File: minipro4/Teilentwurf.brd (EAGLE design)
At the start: 105.1 x 94.6 mm, 91 parts, among them IC1 MEGA8-P, IC2 FT232RL_ADAPTER, IC3 78L08Z, IC4 4051N, IC5 TL082P, IC6 4051N, IC7 TL082P, J1 HOHLSTECKER, Q2 BS170, Q3 BS170, Q4 BS170, Q6 IRF4905, X1 , X2 CON_COAX

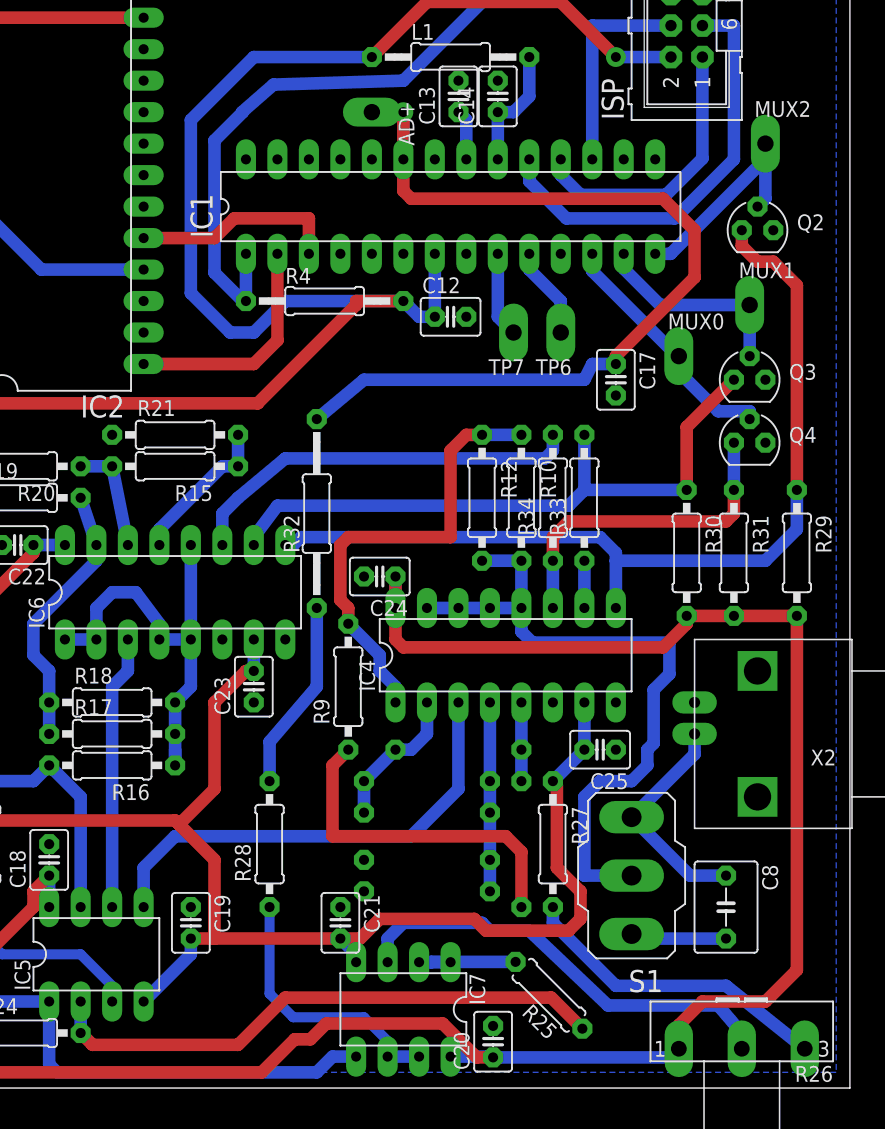
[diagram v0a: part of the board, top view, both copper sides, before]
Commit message: Winkel überarbeitet
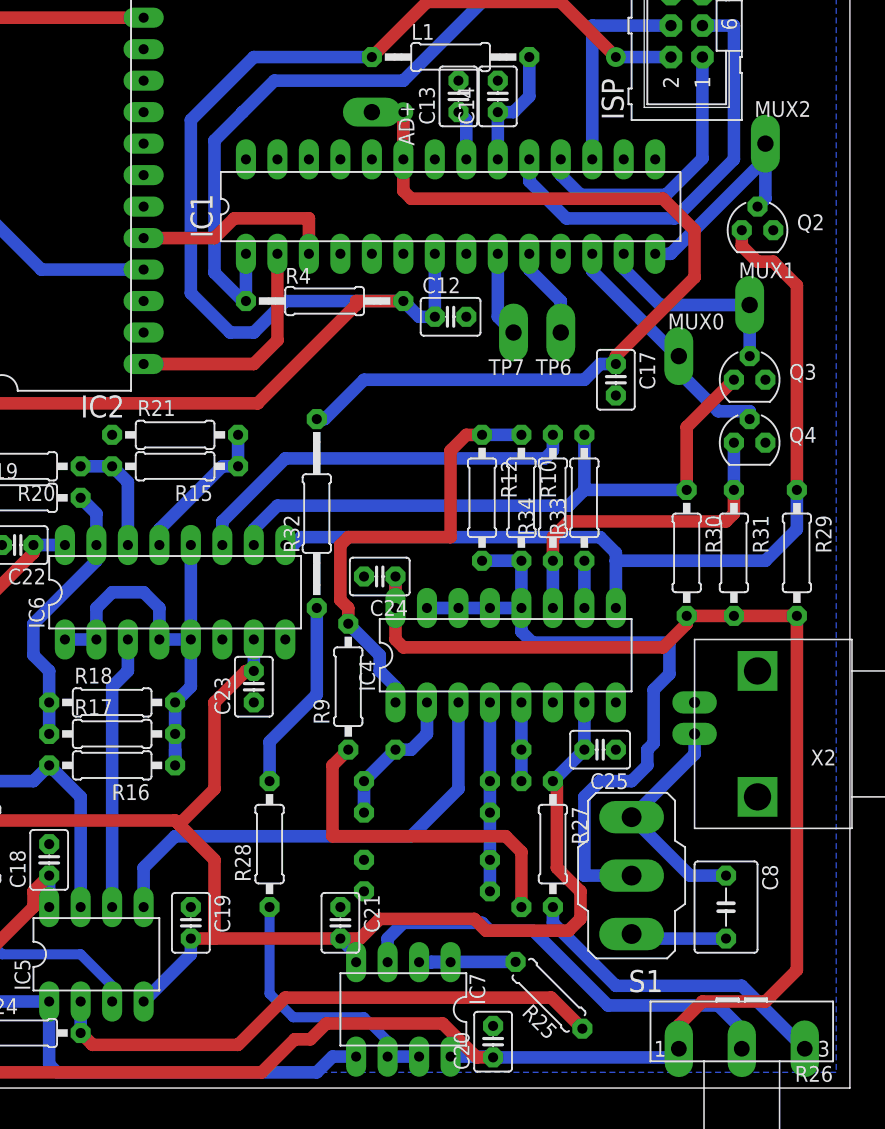
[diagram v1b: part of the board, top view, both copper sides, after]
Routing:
- net N$23: track 35.3 -> 35.9 mm
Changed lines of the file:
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@@
 </class>
 </classes>
-<designrules name="DesignRules_Grounplane">
+<designrules name="DesignRules_Grounplane *">
 <description language="de">&lt;b&gt;EAGLE Design Rules&lt;/b&gt;
 &lt;p&gt;
@@
 <param name="dpGapFactor" value="2.5"/>
 <param name="checkGrid" value="0"/>
-<param name="checkAngle" value="0"/>
+<param name="checkAngle" value="1"/>
 <param name="checkFont" value="1"/>
 <param name="checkRestrict" value="1"/>
@@
 <contactref element="C17" pad="1"/>
 <wire x1="92.71" y1="67.31" x2="92.71" y2="63.5" width="1.016" layer="1"/>
-<wire x1="62.23" y1="52.07" x2="66.04" y2="55.245" width="1.016" layer="16"/>
 <wire x1="66.04" y1="55.245" x2="83.82" y2="55.245" width="1.016" layer="16"/>
-<wire x1="83.82" y1="55.245" x2="84.455" y2="56.515" width="1.016" layer="16"/>
-<wire x1="84.455" y1="56.515" x2="86.36" y2="56.515" width="1.016" layer="16"/>
 <wire x1="86.36" y1="56.515" x2="86.36" y2="57.15" width="1.016" layer="1"/>
 <wire x1="86.36" y1="57.15" x2="92.71" y2="63.5" width="1.016" layer="1"/>
@@
 <wire x1="69.215" y1="73.025" x2="69.215" y2="76.835" width="1.016" layer="1"/>
 <via x="69.215" y="76.835" extent="1-16" drill="0.8" shape="square"/>
+<wire x1="66.04" y1="55.245" x2="62.865" y2="52.07" width="1.016" layer="16"/>
+<wire x1="62.865" y1="52.07" x2="62.23" y2="52.07" width="1.016" layer="16"/>
+<wire x1="86.36" y1="56.515" x2="85.09" y2="56.515" width="1.016" layer="16"/>
+<wire x1="85.09" y1="56.515" x2="83.82" y2="55.245" width="1.016" layer="16"/>
 </signal>
 <signal name="MUX0">
@@
 <wire x1="56.2645" y1="61.595" x2="53.975" y2="63.8845" width="1.016" layer="16"/>
 <wire x1="53.975" y1="63.8845" x2="53.975" y2="74.5455" width="1.016" layer="16"/>
-<wire x1="53.975" y1="74.5455" x2="56.2645" y2="76.835" width="1.016" layer="16"/>
 <wire x1="78.74" y1="88.9" x2="91.549" y2="88.9" width="1.016" layer="16"/>
 <wire x1="91.549" y1="88.9" x2="93.345" y2="87.104" width="1.016" layer="16"/>
 <wire x1="93.345" y1="87.104" x2="93.345" y2="86.36" width="1.016" layer="16"/>
 <wire x1="56.2645" y1="76.835" x2="56.1975" y2="76.835" width="1.016" layer="16"/>
-<wire x1="56.1975" y1="76.835" x2="58.7375" y2="79.0575" width="1.016" layer="16"/>
-<wire x1="58.7375" y1="79.0575" x2="69.215" y2="79.375" width="1.016" layer="16"/>
 <wire x1="69.215" y1="79.375" x2="78.74" y2="88.9" width="1.016" layer="16"/>
+<wire x1="69.215" y1="79.375" x2="58.8045" y2="79.375" width="1.016" layer="16"/>
+<wire x1="58.8045" y1="79.375" x2="53.975" y2="74.5455" width="1.016" layer="16"/>
+<wire x1="53.975" y1="74.5455" x2="56.1975" y2="76.835" width="0" layer="19" extent="16-16"/>
 </signal>
 <signal name="N$5">
@@
 <contactref element="IC6" pad="10"/>
 <contactref element="R33" pad="2"/>
-<wire x1="57.15" y1="41.91" x2="57.15" y2="42.545" width="1.016" layer="16"/>
-<wire x1="57.15" y1="42.545" x2="59.055" y2="45.085" width="1.016" layer="16"/>
 <wire x1="59.055" y1="45.085" x2="82.55" y2="45.085" width="1.016" layer="16"/>
 <wire x1="82.55" y1="45.085" x2="83.82" y2="46.355" width="1.016" layer="16"/>
 <wire x1="83.82" y1="46.355" x2="83.82" y2="50.8" width="1.016" layer="16"/>
 <wire x1="92.075" y1="46.355" x2="83.82" y2="46.355" width="1.016" layer="16"/>
+<wire x1="57.15" y1="41.91" x2="57.15" y2="43.18" width="1.016" layer="16"/>
+<wire x1="57.15" y1="43.18" x2="59.055" y2="45.085" width="1.016" layer="16"/>
 </signal>
 <signal name="MUX2*">
@@
 <contactref element="IC6" pad="14"/>
 <wire x1="43.18" y1="48.26" x2="45.72" y2="48.26" width="1.016" layer="16"/>
-<wire x1="45.72" y1="48.26" x2="46.99" y2="41.91" width="1.016" layer="16"/>
+<wire x1="46.99" y1="41.91" x2="46.99" y2="46.99" width="1.016" layer="16"/>
+<wire x1="46.99" y1="46.99" x2="45.72" y2="48.26" width="1.016" layer="16"/>
 </signal>
 <signal name="N$33">
@@
 <contactref element="R18" pad="1"/>
 <contactref element="IC6" pad="15"/>
-<wire x1="43.18" y1="45.72" x2="44.45" y2="41.91" width="1.016" layer="16"/>
 <wire x1="40.64" y1="29.21" x2="40.64" y2="26.67" width="1.016" layer="16"/>
 <wire x1="40.64" y1="29.21" x2="40.64" y2="31.75" width="1.016" layer="16"/>
@@
 <wire x1="39.37" y1="35.56" x2="44.45" y2="40.64" width="1.016" layer="16"/>
 <wire x1="44.45" y1="40.64" x2="44.45" y2="41.91" width="1.016" layer="16"/>
+<wire x1="44.45" y1="41.91" x2="44.45" y2="44.45" width="1.016" layer="16"/>
+<wire x1="44.45" y1="44.45" x2="43.18" y2="45.72" width="1.016" layer="16"/>
 </signal>
 <signal name="N$34">
@@
 <wire x1="81.28" y1="12.7" x2="81.28" y2="11.43" width="1.016" layer="16"/>
 <wire x1="81.28" y1="11.43" x2="86.36" y2="6.35" width="1.016" layer="16"/>
-<wire x1="95.25" y1="6.35" x2="101.6" y2="1.27" width="1.016" layer="16"/>
-<wire x1="86.36" y1="6.35" x2="95.25" y2="6.35" width="1.016" layer="16"/>
+<wire x1="86.36" y1="6.35" x2="96.52" y2="6.35" width="1.016" layer="16"/>
+<wire x1="96.52" y1="6.35" x2="101.6" y2="1.27" width="1.016" layer="16"/>
 </signal>
 <signal name="N$39">
@@
 <wire x1="67.945" y1="8.255" x2="67.945" y2="10.16" width="1.016" layer="16"/>
 <wire x1="67.945" y1="10.16" x2="69.215" y2="11.43" width="1.016" layer="16"/>
-<wire x1="96.52" y1="1.27" x2="96.52" y2="2.54" width="1.016" layer="16"/>
-<wire x1="96.52" y1="2.54" x2="94.615" y2="4.7625" width="1.016" layer="16"/>
+<wire x1="96.52" y1="1.27" x2="96.52" y2="1.905" width="1.016" layer="16"/>
+<wire x1="96.52" y1="1.905" x2="96.52" y2="2.54" width="1.016" layer="16"/>
 <wire x1="94.615" y1="4.7625" x2="85.725" y2="4.7625" width="1.016" layer="16"/>
-<wire x1="85.725" y1="4.7625" x2="79.375" y2="10.795" width="1.016" layer="16"/>
-<wire x1="79.375" y1="10.795" x2="76.2" y2="10.795" width="1.016" layer="16"/>
 <wire x1="76.2" y1="10.795" x2="75.565" y2="11.43" width="1.016" layer="16"/>
 <wire x1="75.565" y1="11.43" x2="69.215" y2="11.43" width="1.016" layer="16"/>
+<wire x1="76.2" y1="10.795" x2="79.6925" y2="10.795" width="1.016" layer="16"/>
+<wire x1="79.6925" y1="10.795" x2="85.725" y2="4.7625" width="1.016" layer="16"/>
+<wire x1="94.615" y1="4.7625" x2="96.52" y2="2.8575" width="1.016" layer="16"/>
+<wire x1="96.52" y1="2.8575" x2="96.52" y2="2.54" width="1.016" layer="16"/>
 </signal>
 <signal name="N$40">
@@
 <contactref element="R28" pad="2"/>
 <contactref element="R32" pad="1"/>
-<wire x1="58.42" y1="22.86" x2="58.42" y2="26.035" width="1.016" layer="16"/>
-<wire x1="58.42" y1="26.035" x2="62.23" y2="30.48" width="1.016" layer="16"/>
-<wire x1="62.23" y1="30.48" x2="62.23" y2="36.83" width="1.016" layer="16"/>
+<wire x1="62.23" y1="29.845" x2="62.23" y2="36.83" width="1.016" layer="16"/>
+<wire x1="62.23" y1="29.845" x2="58.42" y2="26.035" width="1.016" layer="16"/>
+<wire x1="58.42" y1="26.035" x2="58.42" y2="22.86" width="1.016" layer="16"/>
 </signal>
 <signal name="N$23">
@@
 <wire x1="52.07" y1="34.29" x2="52.07" y2="41.91" width="1.016" layer="16"/>
 <wire x1="41.91" y1="34.29" x2="44.45" y2="34.29" width="1.016" layer="16"/>
-<wire x1="49.53" y1="35.56" x2="49.53" y2="34.29" width="1.016" layer="16"/>
 <wire x1="49.53" y1="34.29" x2="52.07" y2="34.29" width="1.016" layer="16"/>
 <wire x1="50.8" y1="25.4" x2="50.8" y2="24.13" width="1.016" layer="16"/>
@@
 <wire x1="44.45" y1="34.29" x2="44.45" y2="36.83" width="1.016" layer="16"/>
 <wire x1="44.45" y1="36.83" x2="45.72" y2="38.1" width="1.016" layer="16"/>
-<wire x1="45.72" y1="38.1" x2="47.625" y2="38.1" width="1.016" layer="16"/>
-<wire x1="47.625" y1="38.1" x2="49.53" y2="35.56" width="1.016" layer="16"/>
+<wire x1="49.53" y1="34.29" x2="49.53" y2="36.83" width="1.016" layer="16"/>
+<wire x1="49.53" y1="36.83" x2="48.26" y2="38.1" width="1.016" layer="16"/>
+<wire x1="48.26" y1="38.1" x2="45.72" y2="38.1" width="1.016" layer="16"/>
 </signal>
 <signal name="N$45">
@@
 <wire x1="81.28" y1="49.53" x2="80.645" y2="48.895" width="1.016" layer="16"/>
 <wire x1="80.645" y1="48.895" x2="59.69" y2="48.895" width="1.016" layer="16"/>
-<wire x1="59.69" y1="48.895" x2="55.88" y2="45.72" width="1.016" layer="16"/>
-<wire x1="55.88" y1="45.72" x2="54.61" y2="44.45" width="1.016" layer="16"/>
-<wire x1="54.61" y1="44.45" x2="54.61" y2="41.91" width="1.016" layer="16"/>
+<wire x1="54.61" y1="41.91" x2="54.61" y2="43.815" width="1.016" layer="16"/>
+<wire x1="54.61" y1="43.815" x2="59.69" y2="48.895" width="1.016" layer="16"/>
 </signal>
 <signal name="MUX1*A">
